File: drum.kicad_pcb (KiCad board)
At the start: 4 copper layers, 70 x 70 mm, 112 parts, among them J1001 NE8FAV, J101 Cortex, J102 DX07S016JA3, J501 WAGO 2065-100, J502 WAGO 2065-100, J601 WAGO 2065-100, J602 WAGO 2065-100, J701 WAGO 2065-100, J702 WAGO 2065-100, J703 WAGO 2065-100, J704 WAGO 2065-100, J801 WAGO 2065-100, J802 WAGO 2065-100, J803 WAGO 2065-100, J901 NE8FAV, Q201 BSC010N04LS, Q202 BSC010N04LS, Q501 BSC010N04LS, Q601 BSC010N04LS, SW101 SKSG, SW102 SKSG, U1001 THVD2442, U101 ATSAMD51J, U102 TPS78433QWDRBRQ1, U201 LM74502-Q1, U301 TPSM33625, U401 BTT6010, U701 TMC2130-LA, U801 74AHC1G125, U901 THVD2442, Y101 32k768

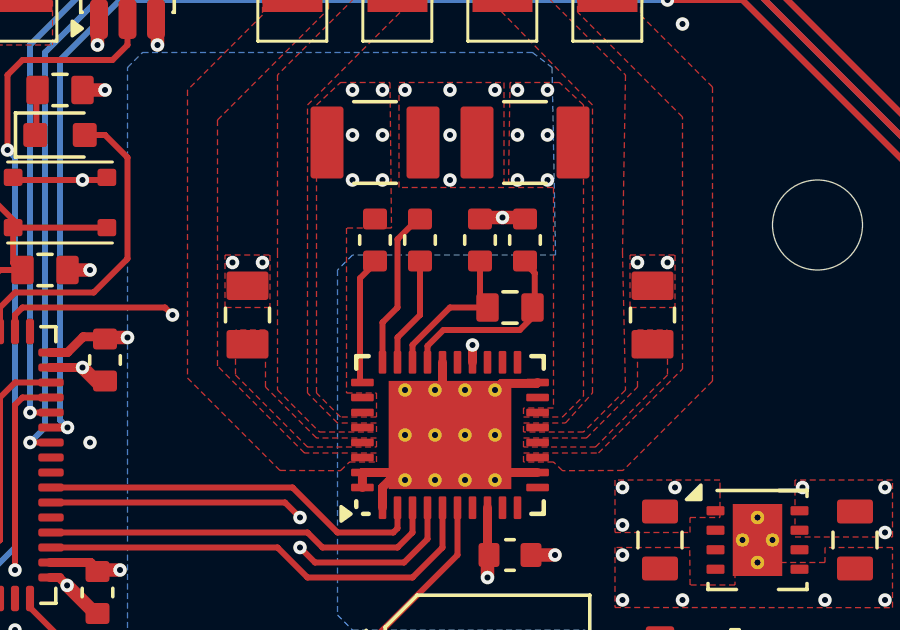
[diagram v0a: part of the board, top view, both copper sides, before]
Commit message: Use date as revision
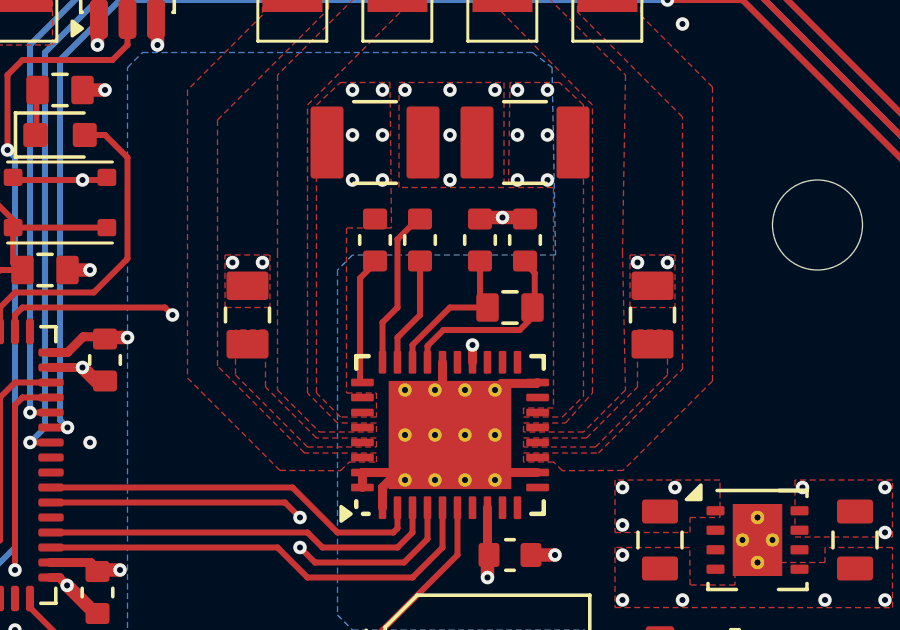
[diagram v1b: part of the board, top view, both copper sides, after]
